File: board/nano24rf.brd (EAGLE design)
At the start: 17.8 x 50 mm, 26 parts, among them CN1 1X4-CLEANBIG, CN2 1X4-CLEANBIG, CN3 1X4-CLEANBIG, CN4 1X4-CLEANBIG

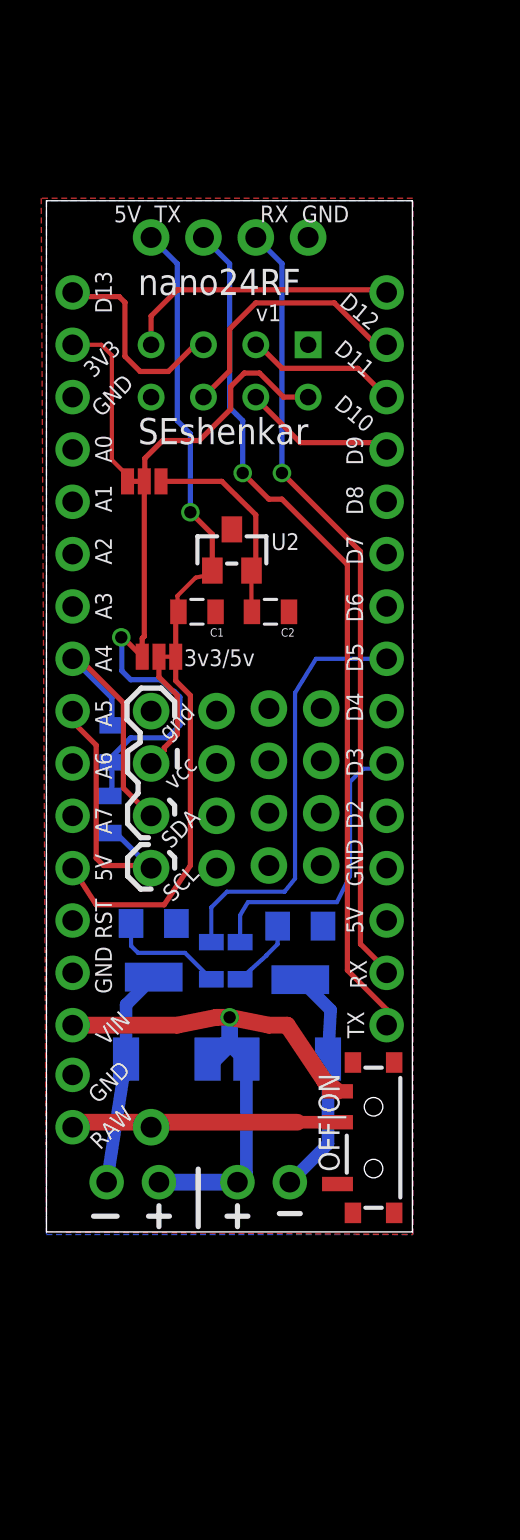
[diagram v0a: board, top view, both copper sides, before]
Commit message: before route
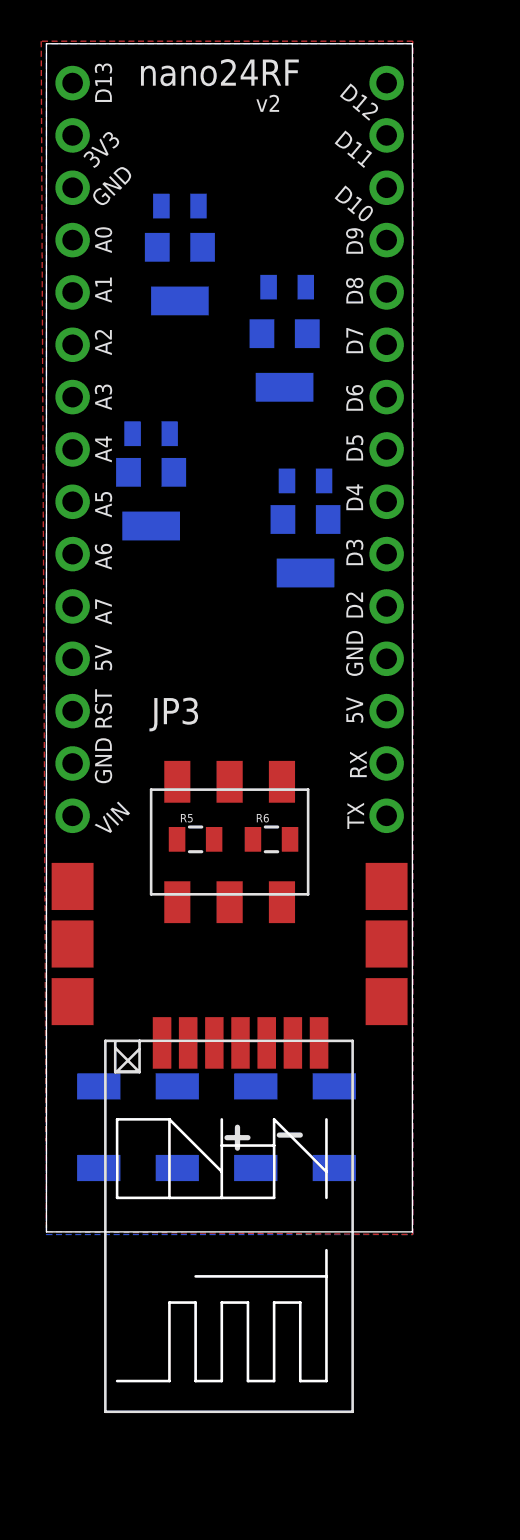
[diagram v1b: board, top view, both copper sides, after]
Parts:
- removed C1, C2: (no value), ATTAMI-V0.00:0805
- removed CN1, CN2, CN3, CN4, I2CPORT: 1X4-CLEANBIG, adafruit:1X04-CLEANBIG
- removed FET1, FET2, JP6: (no value), ATTAMI-V0.00:1X02_ROUND
- removed SJ1: JUMPER-PAD-3-2OF3_NC_BY_TRACE_SMALL, ATTAMI-V0.00:PAD-JUMPER-3-2OF3_NC_BY_TRACE_YES_SILK_FULL_BOX
- removed SJ2: (no value), ATTAMI-V0.00:PAD-JUMPER-3-2OF3_NC_BY_TRACE_YES_SILK_FULL_BOX
- removed SW1: (no value), microbuilder:SPST_SMT_19192
- removed U$2: NRF24, ATTAMI-V0.00:NRF24-2X4
- removed U2: (no value), microbuilder:SOT23-WIDE
- added D3, D4: (no value), dp_devices:DO-214AC
- added Q3, Q4: (no value), adafruit:SOT23-W
- added R5, R6: (no value), ATTAMI-V0.00:0805
- added U$6, U$8: 1X3SMD, nanorf24:FATPAD
- added U$7: 1X7-SMDPADS, nanorf24:SMD1,27-2,54
- JP3: device adafruit:1X01-CLEANBIG -> pinhead+:2X03_SMT
- moved R4 27.0 mm to (11.7, 45.8), turned to 0 degrees
- moved R3 26.3 mm to (6.48, 49.8), turned to 0 degrees
- moved R1 25.9 mm to (5.08, 38.7), turned to 0 degrees
- moved R2 23.7 mm to (12.6, 36.4), turned to 0 degrees
- moved Q1 23.2 mm to (5.08, 35.6)
- moved Q2 20.9 mm to (12.6, 33.3)
- moved JP3 14.4 mm to (8.89, 18.9)
- moved JP1 10.2 mm to (1.27, 38.0)
- moved JP2 10.2 mm to (16.5, 38.0)
- moved D2 5.44 mm to (10.2, 5.08), turned to 90 degrees
- moved D1 4.02 mm to (14.0, 5.08), turned to 90 degrees
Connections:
- removed net IRQ: U$2.IRQ
- removed net N$1 (its old number): D1.2, FET1.2, Q1.3
- removed net RAW: JP3.1, JP6.1, SW1.B
- removed net RX: CN4.3, JP2.14
- removed net TX: CN4.2, JP2.15
- removed net V-ADJ: C2.1, SJ1.1, U2.2
- removed net V-NRF: SJ1.2, U$2.VCC
- new net D10: JP2.3, R3.1
- new net D9: JP2.4, R4.1
- new net FET01: D1.2, Q1.3, U$8.P$1
- new net FET02: D2.2, Q2.3, U$8.P$3
- new net FET03: D3.2, Q3.3, U$6.P$1
- new net FET04: D4.2, Q4.3, U$6.P$3
- new net N$5: Q4.1, R4.2
- net 3V3: no longer R3.2, R4.2, SJ1.3, SJ2.1
- net 5V: now also JP3.2, R5.1; no longer C1.1, CN4.1, JP1.12, SJ2.3, U2.1
- net CE: now also JP2.6, U$7.2; no longer JP2.3, U$2.CE
- net CSN: now also JP2.5, U$7.3; no longer JP2.4, U$2.CSN
- net D3: no longer R1.1
- net D6: now also R1.1
- net GND: now also JP3.6, Q3.2, Q4.2, R6.1, U$7.4; no longer C1.2, C2.2, CN4.4, I2CPORT.4, JP6.2, U$2.GND, U2.3
- net MISO: now also JP3.1, U$7.5; no longer JP2.1, U$2.MISO
- net MOSI: now also JP3.4, U$7.6; no longer JP2.2, U$2.MOSI
- net N$4: now also Q3.1, R3.2; no longer D2.2, FET2.2, Q2.3
- net N$6: now also R5.2, R6.2, U$7.1; no longer I2CPORT.3, SJ2.2
- net RST: now also JP3.5; no longer JP2.13
- net SCK: now also JP3.3, U$7.7; no longer JP1.1, U$2.SCK
- net SCL: no longer I2CPORT.1, R4.1
- net SDA: no longer I2CPORT.2, R3.1
- net VIN: now also D3.1, D4.1, U$6.P$2, U$8.P$2; no longer FET1.1, FET2.1, SW1.C
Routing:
- net TX: track 42.3 -> 0.00 mm, vias 1 -> 0
- net 5V: track 41.4 -> 0.00 mm, vias 1 -> 0
- net RX: track 38.3 -> 0.00 mm, vias 1 -> 0
- net 3V3: track 31.5 -> 0.00 mm, vias 1 -> 0
- net VIN: track 29.5 -> 0.00 mm, vias 1 -> 0
- net D5: track 20.8 -> 0.00 mm
- net RAW: track 16.6 -> 0.00 mm
- net D3: track 14.5 -> 0.00 mm
- net SDA: track 13.4 -> 0.00 mm
- net MISO: track 13.4 -> 0.00 mm
- net SCL: track 13.2 -> 0.00 mm
- net MOSI: track 12.8 -> 0.00 mm
- net V-NRF: track 11.9 -> 0.00 mm
- net N$1 (its old number): track 11.4 -> 0.00 mm
- net N$4: track 10.7 -> 0.00 mm
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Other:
- board size 17.8 x 50 mm -> 17.8 x 57.7 mm
- board text added: "v2"
- board text removed: "3v3/5v"
- board text removed: "5V TX RX GND"
- board text removed: "OFF|ON"
- board text removed: "RAW"
- board text removed: "SCL"
- board text removed: "SDA"
- board text removed: "SEshenkar"
- board text removed: "gnd"
- board text removed: "this way"
- board text removed: "v1"
- board text removed: "vcc"

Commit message: added lib, need to fix volt div placment
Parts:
- JP3: device pinhead+:2X03_SMT -> nano24rf:2X03_SMT
- U$7: device nanorf24:SMD1,27-2,54 -> nano24rf:SMD1,27-2,54
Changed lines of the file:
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@@
 <attribute name="VALUE" x="13.335" y="57.023" size="0.4064" layer="27" ratio="10" rot="R270"/>
 </element>
-<element name="JP3" library="pinhead+" package="2X03_SMT" value="" x="8.89" y="18.923"/>
-<element name="U$7" library="nanorf24" package="SMD1,27-2,54" value="1X7-SMDPADS" x="14.859" y="9.271" smashed="yes" rot="R180"/>
+<element name="JP3" library="nano24rf" package="2X03_SMT" value="" x="8.89" y="18.923"/>
+<element name="U$7" library="nano24rf" package="SMD1,27-2,54" value="1X7-SMDPADS" x="14.859" y="9.271" smashed="yes" rot="R180"/>
 <element name="Q2" library="adafruit" package="SOT23-W" value="" x="12.573" y="33.274" smashed="yes" rot="MR180">
 <attribute name="VALUE" x="14.605" y="33.782" size="0.4064" layer="28" rot="MR180"/>

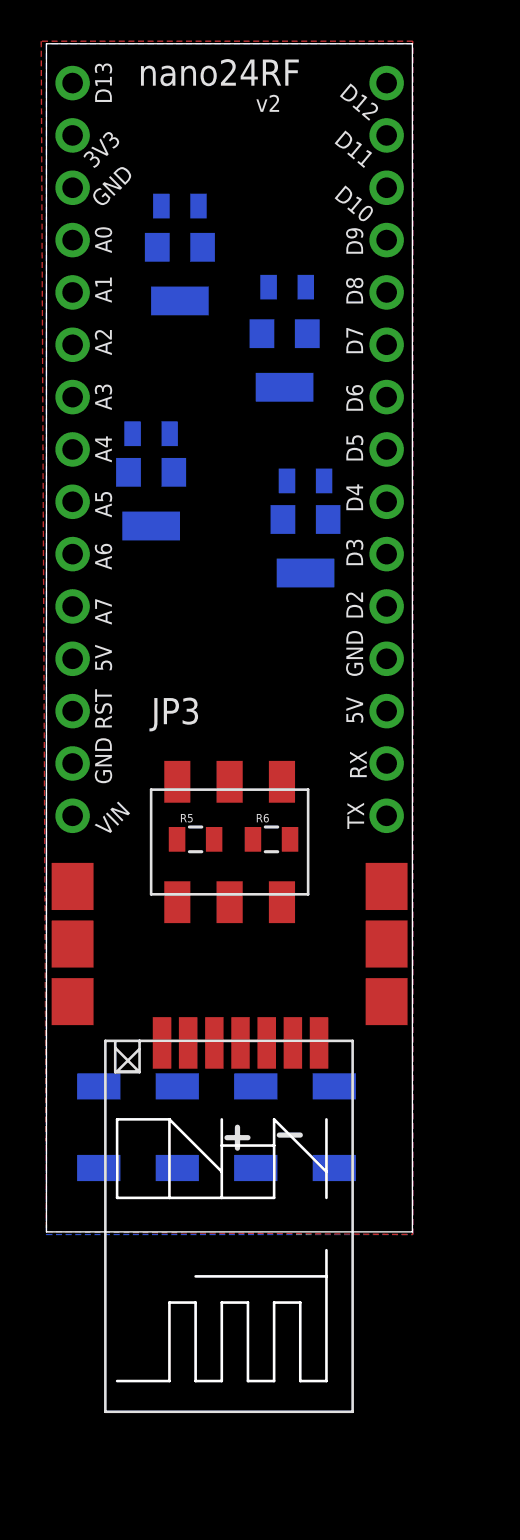
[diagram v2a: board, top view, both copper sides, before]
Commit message: ready to grb
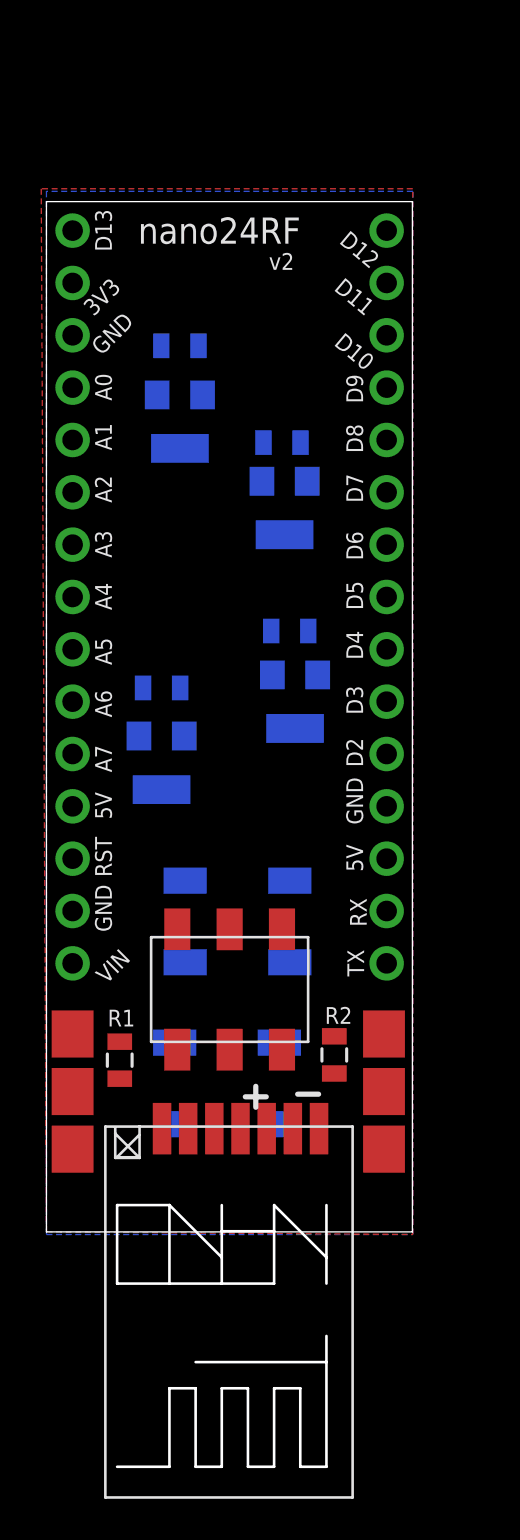
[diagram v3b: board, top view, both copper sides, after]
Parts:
- moved R1 30.4 mm to (3.56, 8.33), flipped to the top, turned to 270 degrees
- moved R2 27.9 mm to (14.0, 8.59), flipped to the top, turned to 270 degrees
- moved R5 24.0 mm to (6.48, 43.0), flipped to the bottom
- moved R3 23.4 mm to (5.59, 26.4), turned to 180 degrees
- moved R6 19.3 mm to (11.4, 38.3), flipped to the bottom
- moved R4 16.7 mm to (11.8, 29.2)
- moved Q1 12.8 mm to (5.59, 22.8)
- moved D2 10.1 mm to (11.8, 15.1)
- moved D4 9.99 mm to (6.73, 15.1)
- moved Q2 7.56 mm to (12.1, 25.7)
- moved U$8 7.16 mm to (16.4, 6.81)
- moved U$6 7.16 mm to (1.27, 6.81)
- moved JP1 7.16 mm to (1.27, 30.8)
- moved JP2 7.16 mm to (16.5, 30.8)
- moved JP3 7.16 mm to (8.89, 11.8)
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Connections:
- removed net N$1: Q2.1, R2.2
- removed net N$2: Q1.1, R1.2
- removed net N$4: Q3.1, R3.2
- removed net N$5: Q4.1, R4.2
- net 5V: now also R1.1; no longer R5.1
- net D10: now also Q3.1, R5.2; no longer R3.1
- net D5: now also Q2.1, R4.2; no longer R2.1
- net D6: now also Q1.1, R3.2; no longer R1.1
- net D9: now also Q4.1, R6.2; no longer R4.1
- net GND: now also R2.1, R3.1, R4.1, R5.1
- net N$6: now also R1.2, R2.2; no longer R5.2, R6.2
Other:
- board size 17.8 x 57.7 mm -> 17.8 x 50 mm
